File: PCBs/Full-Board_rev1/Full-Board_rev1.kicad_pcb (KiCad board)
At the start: 2 copper layers, 30 parts, among them J1 TYPE-C-31-M-12, J10 Conn_01x11, J11 Conn_01x02_Pin, J12 Conn_01x02, J13 Conn_01x04, J2 Conn_01x05, J3 Conn_01x05, J4 Conn_01x05, J5 Conn_01x05, J6 MotorWithEncoder_M2, J7 MotorWithEncoder_M1, J8 Conn_01x02_Batt, J9 Conn_01x02_Batt, Q2 ESP32-C6-WROOM-1

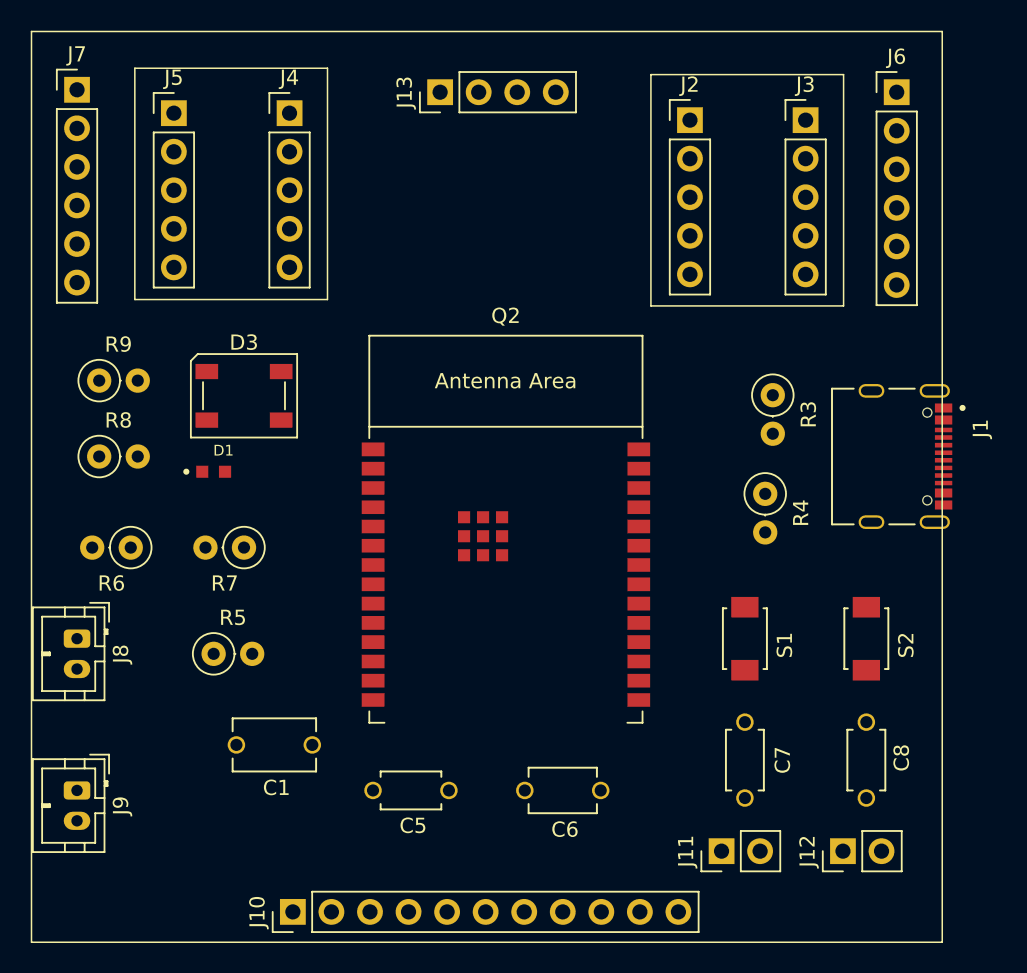
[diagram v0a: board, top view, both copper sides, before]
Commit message: Full Board PCB Design Rev1.0 complete
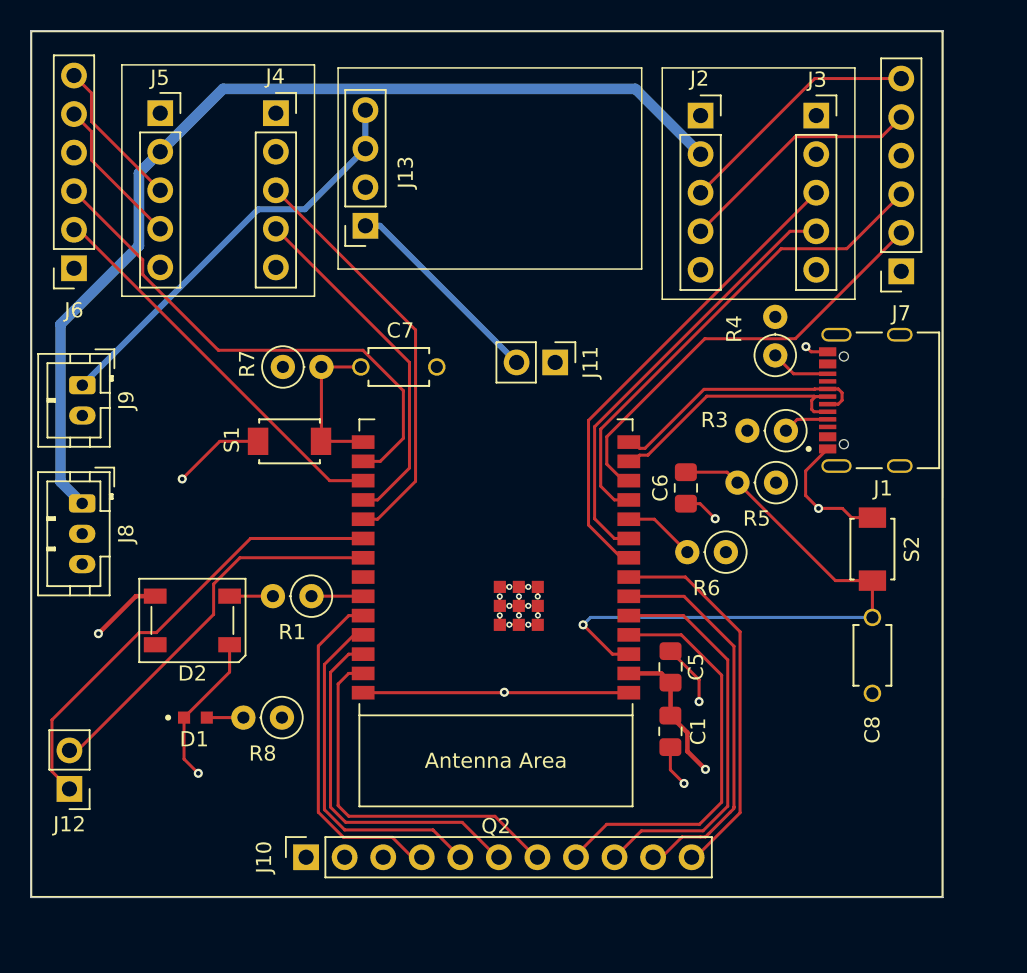
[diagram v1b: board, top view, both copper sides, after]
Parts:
- removed D3: SK6812, LED_SMD:LED_SK6812_PLCC4_5.0x5.0mm_P3.2mm
- removed R9: R, Resistor_THT:R_Axial_DIN0207_L6.3mm_D2.5mm_P2.54mm_Vertical
- added D2: SK6812, LED_SMD:LED_SK6812_PLCC4_5.0x5.0mm_P3.2mm, F.Cu at (122.6, 91.8)
- added R1: R, Resistor_THT:R_Axial_DIN0207_L6.3mm_D2.5mm_P2.54mm_Vertical, F.Cu at (130.4, 90.2)
- C1: footprint 10uCap:CAPRB500W50L550T350H600 -> Capacitor_SMD:C_0805_2012Metric_Pad1.18x1.45mm_HandSolder
- C5: footprint 100nCap:CAPRB500W50L400T250H550 -> Capacitor_SMD:C_0805_2012Metric_Pad1.18x1.45mm_HandSolder
- C6: footprint 1uCap:CAPRB500W50L450T300H550 -> Capacitor_SMD:C_0805_2012Metric_Pad1.18x1.45mm_HandSolder
- J10: footprint Connector_PinHeader_2.54mm:PinHeader_1x11_P2.54mm_Vertical -> Connector_PinSocket_2.54mm:PinSocket_1x11_P2.54mm_Vertical
- J13: footprint Connector_PinHeader_2.54mm:PinHeader_1x04_P2.54mm_Vertical -> Connector_PinSocket_2.54mm:PinSocket_1x04_P2.54mm_Vertical
- J2, J3, J4, J5: footprint Connector_PinHeader_2.54mm:PinHeader_1x05_P2.54mm_Vertical -> Connector_PinSocket_2.54mm:PinSocket_1x05_P2.54mm_Vertical
- J6, J7: footprint Connector_PinHeader_2.54mm:PinHeader_1x06_P2.54mm_Vertical -> Connector_PinSocket_2.54mm:PinSocket_1x06_P2.54mm_Vertical
- J8: value Conn_01x02_Batt -> Conn_01x03; footprint Connector_JST:JST_PH_B2B-PH-K_1x02_P2.00mm_Vertical -> Connector_JST:JST_PH_B3B-PH-K_1x03_P2.00mm_Vertical
- moved J7 55.6 mm to (169.3, 68.8), turned to 180 degrees
- moved J6 55.4 mm to (114.8, 68.6), turned to 180 degrees
- moved J12 51.1 mm to (114.5, 102.9), turned to 180 degrees
- moved R6 39.2 mm to (157.7, 87.3)
- moved R5 38.7 mm to (161.1, 82.7), turned to 180 degrees
- moved C7 34.5 mm to (136.2, 75.1), turned to 180 degrees
- moved J11 34.0 mm to (146.5, 74.8), turned to -90 degrees
- moved S1 32.7 mm to (129.0, 80.0), turned to 0 degrees
- moved J9 26.7 mm to (115.3, 76.3)
- moved C1 26.1 mm to (154.1, 99.1), turned to 90 degrees
- moved C6 21.5 mm to (155.1, 83.1), turned to 90 degrees
- moved R8 21.0 mm to (128.5, 98.2), turned to 180 degrees
- moved C5 18.9 mm to (154.1, 94.9), turned to -90 degrees
- moved D1 16.2 mm to (122.8, 98.2)
- moved R7 12.2 mm to (128.6, 75.1), turned to 0 degrees
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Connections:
- Q2 pad 11: /IR_O1 -> /ENC_PH_B_M1
- Q2 pad 12: /IR_O2 -> /ENC_PH_A_M1
- Q2 pad 16: /IR_O4 -> /ENC_PH_B_M2
- Q2 pad 17: /IR_O5 -> /ENC_PH_A_M2
- Q2 pad 18: /IR_O6 -> /M2_PWM_PH
- Q2 pad 19: /IR_O7 -> /M2_PWM_EN
- Q2 pad 20: /IR_O8 -> Net-(J12-Pin_1)
- Q2 pad 21: /Status_LED/LED_GPIO -> Net-(J12-Pin_2)
- Q2 pad 23: /IR_O3 -> /Status_LED/LED_GPIO
- Q2 pad 24: Net-(J12-Pin_2) -> /IR_O1
- Q2 pad 25: Net-(J12-Pin_1) -> /IR_O2
- Q2 pad 26: /ENC_PH_B_M2 -> /IR_O3
- Q2 pad 27: /ENC_PH_A_M2 -> /IR_O4
- Q2 pad 4: /M1_PWM_EN -> /IR_O5
- Q2 pad 5: /M1_PWM_PH -> /IR_O6
- Q2 pad 6: /M2_PWM_EN -> /IR_O7
- Q2 pad 7: /M2_PWM_PH -> /IR_O8
- Q2 pad 8: /ENC_PH_A_M1 -> /M1_PWM_EN
- Q2 pad 9: /ENC_PH_B_M1 -> /M1_PWM_PH
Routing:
- net /6V: track 0.00 -> 65.6 mm
- net GND: track 0.00 -> 60.6 mm, vias 0 -> 20
- net /CHIP_PU: track 0.00 -> 40.9 mm, vias 0 -> 1
- net /ENC_PH_B_M2: track 0.00 -> 34.1 mm
- net /ENC_PH_B_M1: track 0.00 -> 32.2 mm
- net /M1_PWM_EN: track 0.00 -> 31.7 mm
- net Net-(J12-Pin_1): track 0.00 -> 30.5 mm
- net /M1_PWM_PH: track 0.00 -> 28.8 mm
- net /ENC_PH_A_M1: track 0.00 -> 28.7 mm
- net /VIN: track 0.00 -> 27.6 mm
- net /M2_PWM_EN: track 0.00 -> 27.5 mm
- net /IR_O5: track 0.00 -> 27.4 mm
- net /IR_O6: track 0.00 -> 26.8 mm
- net /IR_O7: track 0.00 -> 25.9 mm
- net /ENC_PH_A_M2: track 0.00 -> 25.9 mm
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- added copper zone on In2.Cu, net /3V3
- added copper zone on In1.Cu, net GND
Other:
- board outline added: 60.1 x 57.1 mm
- copper layers 2 -> 4

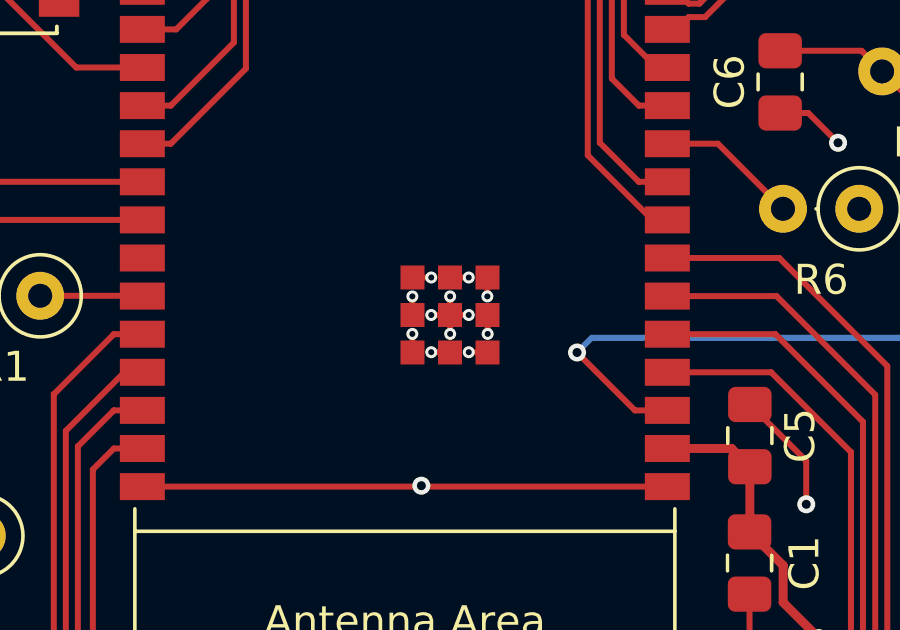
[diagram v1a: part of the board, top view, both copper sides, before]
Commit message: Full Board PCB Design Rev1.1 complete
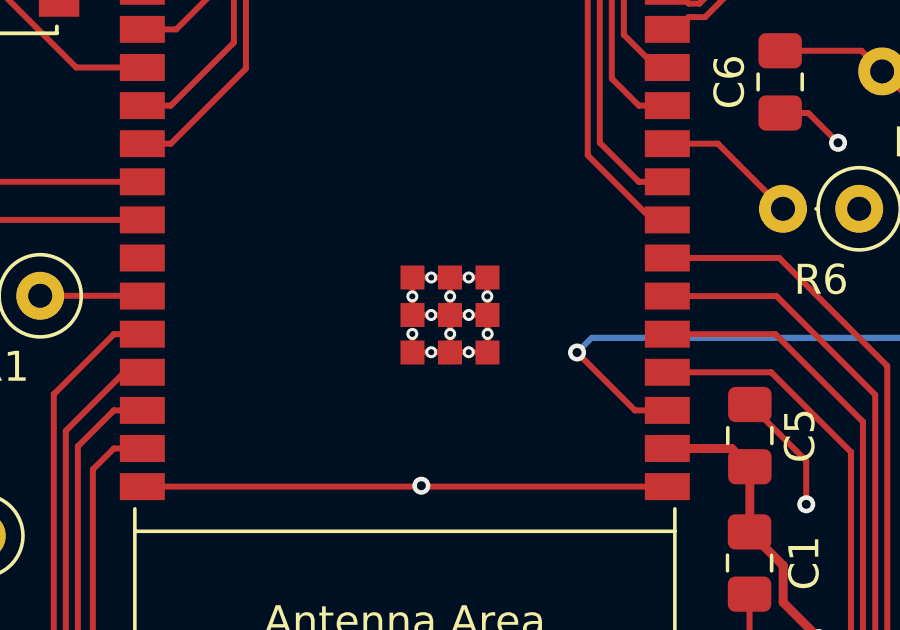
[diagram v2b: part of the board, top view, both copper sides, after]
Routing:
- net GND: track 60.6 -> 67.5 mm
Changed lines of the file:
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@@
+	)
+	(segment
+		(start 145.36 92.085)
+		(end 145.355 92.09)
+		(width 0.2)
+		(layer "F.Cu")
+		(net 2)
 	)
 	(segment
@@
 	)
 	(segment
+		(start 143.48 89.59)
+		(end 144.105 89.59)
+		(width 0.2)
+		(layer "F.Cu")
+		(net 2)
+	)
+	(segment
+		(start 144.11 89.595)
+		(end 144.105 89.59)
+		(width 0.2)
+		(layer "F.Cu")
+		(net 2)
+	)
+	(segment
 		(start 142.85 91.47)
 		(end 142.85 92.085)
@@
 	)
 	(segment
+		(start 144.11 92.085)
+		(end 144.105 92.09)
+		(width 0.2)
+		(layer "F.Cu")
+		(net 2)
+	)
+	(segment
+		(start 143.48 92.08)
+		(end 142.865 92.08)
+		(width 0.2)
+		(layer "F.Cu")
+		(net 2)
+	)
+	(segment
 		(start 144.11 90.22)
 		(end 144.11 90.835)
@@
 	)
 	(segment
+		(start 144.115 92.08)
+		(end 144.105 92.09)
+		(width 0.2)
+		(layer "F.Cu")
+		(net 2)
+	)
+	(segment
+		(start 144.73 89.59)
+		(end 145.355 89.59)
+		(width 0.2)
+		(layer "F.Cu")
+		(net 2)
+	)
+	(segment
 		(start 144.11 90.835)
 		(end 144.105 90.84)
@@
 	)
 	(segment
+		(start 145.35 90.22)
+		(end 145.35 90.835)
+		(width 0.2)
+		(layer "F.Cu")
+		(net 2)
+	)
+	(segment
 		(start 122.05 98.2)
 		(end 122.05 100.93)
@@
 	)
 	(segment
+		(start 142.85 90.22)
+		(end 142.85 89.595)
+		(width 0.2)
+		(layer "F.Cu")
+		(net 2)
+	)
+	(segment
+		(start 143.48 90.84)
+		(end 142.855 90.84)
+		(width 0.2)
+		(layer "F.Cu")
+		(net 2)
+	)
+	(segment
 		(start 125.05 95.2)
 		(end 122.05 98.2)
@@
 	)
 	(segment
+		(start 142.85 89.595)
+		(end 142.855 89.59)
+		(width 0.2)
+		(layer "F.Cu")
+		(net 2)
+	)
+	(segment
 		(start 155.98 95.7025)
 		(end 155.98 97.15)
@@
 	)
 	(segment
+		(start 144.73 92.08)
+		(end 144.115 92.08)
+		(width 0.2)
+		(layer "F.Cu")
+		(net 2)
+	)
+	(segment
 		(start 156.0475 84.1075)
 		(end 157.04 85.1)
@@
 	)
 	(segment
+		(start 145.36 91.47)
+		(end 145.36 92.085)
+		(width 0.2)
+		(layer "F.Cu")
+		(net 2)
+	)
+	(segment
 		(start 126.925 80)
 		(end 124.41 80)
@@
 	)
 	(segment
+		(start 144.11 90.22)
+		(end 144.11 89.595)
+		(width 0.2)
+		(layer "F.Cu")
+		(net 2)
+	)
+	(segment
+		(start 144.73 90.84)
+		(end 145.355 90.84)
+		(width 0.2)
+		(layer "F.Cu")
+		(net 2)
+	)
+	(segment
 		(start 151.35 96.56)
 		(end 143.18 96.56)
@@
 		(width 0.2)
 		(layer "F.Cu")
+		(net 2)
+	)
+	(segment
+		(start 145.35 90.835)
+		(end 145.355 90.84)
+		(width 0.2)
+		(layer "F.Cu")
+		(net 2)
+	)
+	(segment
+		(start 144.11 91.47)
+		(end 144.11 92.085)
+		(width 0.2)
+		(layer "F.Cu")
+		(net 2)
+	)
+	(segment
+		(start 142.865 92.08)
+		(end 142.855 92.09)
+		(width 0.2)
+		(layer "F.Cu")
